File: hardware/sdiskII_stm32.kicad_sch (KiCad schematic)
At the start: 8 parts, among them J2 APPLE_SDISKII, U2 MicroSD_SDIO, U8 DM-OLED096-636

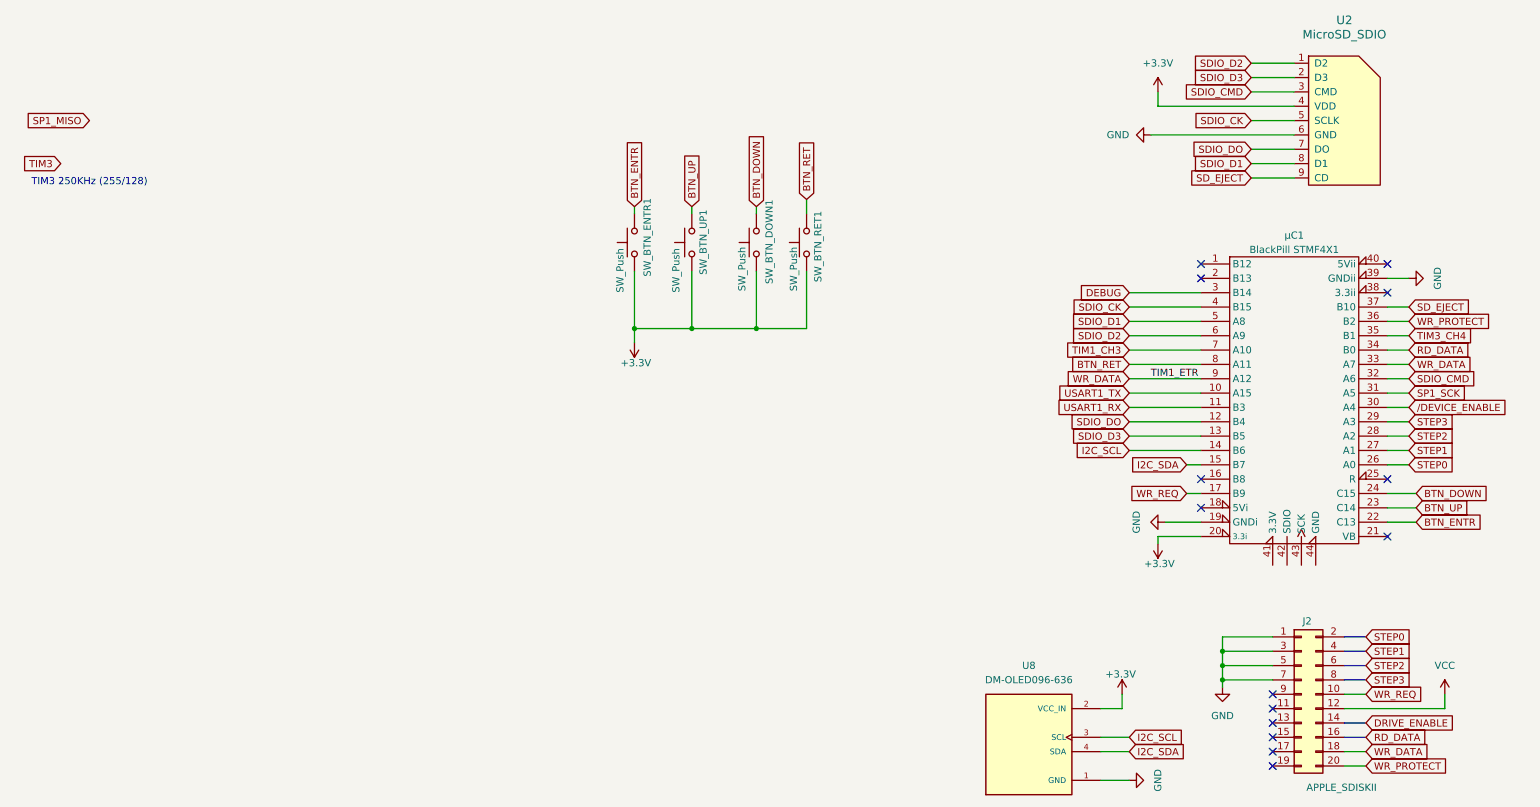
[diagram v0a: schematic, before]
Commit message: new realease with gerber
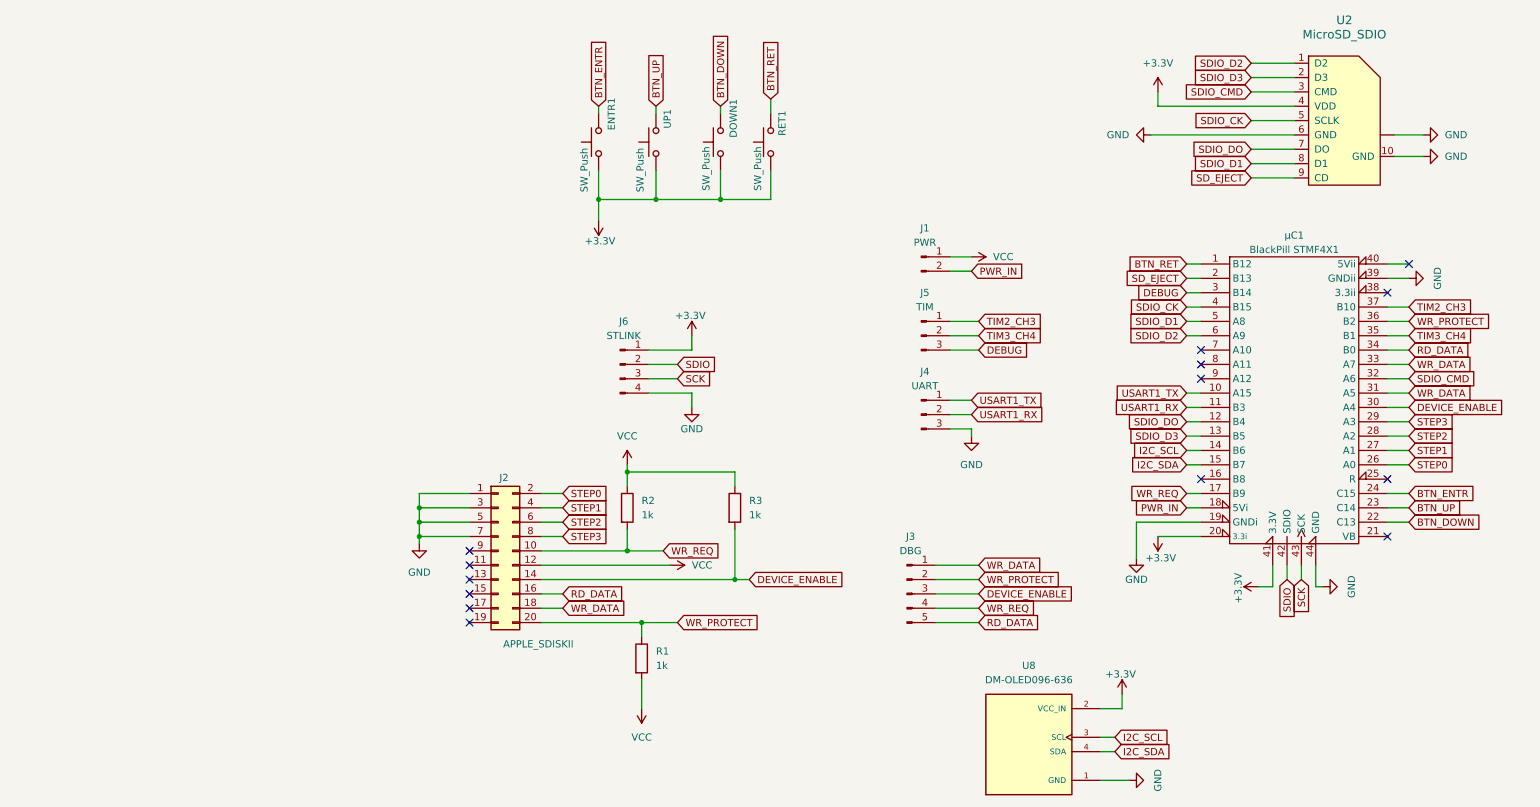
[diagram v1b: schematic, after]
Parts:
- added J1: PWR, Connector_PinHeader_2.54mm:PinHeader_1x02_P2.54mm_Vertical, symbol Connector:Conn_01x02_Pin
- added J3: DBG, Connector_PinHeader_2.54mm:PinHeader_1x05_P2.54mm_Vertical, symbol Connector:Conn_01x05_Pin
- added J4: UART, Connector_PinHeader_2.54mm:PinHeader_1x03_P2.54mm_Vertical, symbol Connector:Conn_01x03_Pin
- added J5: TIM, Connector_PinHeader_2.54mm:PinHeader_1x03_P2.54mm_Vertical, symbol Connector:Conn_01x03_Pin
- added J6: STLINK, Connector_PinHeader_2.54mm:PinHeader_1x04_P2.54mm_Vertical, symbol Connector:Conn_01x04_Pin
- added R1, R2, R3: 1k, Resistor_THT:R_Axial_DIN0207_L6.3mm_D2.5mm_P10.16mm_Horizontal, symbol Device:R
- U2: footprint sdisk_stm32:GCT-MEM2055-00-190-01-A -> sdisk_stm32:GCT-MEM2055-00-190-01-A_VIB
- μC1: footprint acheron_Hardware.pretty-master:Mini_F4X1_STM32 -> acheron_Hardware.pretty-master:Mini_F4X1_STM32_VIB
- renumbered SW_BTN_DOWN1 to DOWN1, SW_BTN_ENTR1 to ENTR1, SW_BTN_RET1 to RET1, SW_BTN_UP1 to UP1
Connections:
- net SP1_SCK is gone; now on net WR_DATA: μC1.31 (A5)
- net /DEVICE_ENABLE is gone; now on net DEVICE_ENABLE: μC1.30 (A4)
- net +3.3V: now also μC1.41 (3.3V), J6.1 (Pin_1)
- net BTN_DOWN: now also μC1.22 (C13); no longer μC1.24 (C15)
- net BTN_ENTR: now also μC1.24 (C15); no longer μC1.22 (C13)
- net BTN_RET: now also μC1.1 (B12); no longer μC1.8 (A11)
- net DEBUG: now also J5.3 (Pin_3)
- net GND: now also U2.10 (GND), U2.~, μC1.44 (GND), J4.3 (Pin_3), J6.4 (Pin_4)
- net RD_DATA: now also J2.16 (Pin_16), J3.5 (Pin_5)
- net SD_EJECT: now also μC1.2 (B13); no longer μC1.37 (B10)
- net STEP0: now also J2.2 (Pin_2)
- net STEP1: now also J2.4 (Pin_4)
- net STEP2: now also J2.6 (Pin_6)
- net STEP3: now also J2.8 (Pin_8)
- net TIM3_CH4: now also J5.2 (Pin_2)
- net USART1_RX: now also J4.2 (Pin_2)
- net USART1_TX: now also J4.1 (Pin_1)
- net VCC: now also J1.1 (Pin_1), R1.2, R2.1, R3.1
- net WR_DATA: now also J3.1 (Pin_1); no longer μC1.9 (A12)
- net WR_PROTECT: now also J3.2 (Pin_2), R1.1
- net WR_REQ: now also J3.4 (Pin_4), R2.2
- net DEVICE_ENABLE: now reaches J2.14 (Pin_14)
- net DEVICE_ENABLE: now also J3.3 (Pin_3), R3.2
- net PWR_IN: now reaches μC1.18 (5Vi)
- net PWR_IN: now also J1.2 (Pin_2)
- net SDIO: now reaches μC1.42 (SDIO)
- net SDIO: now also J6.2 (Pin_2)
- net SCK: now reaches μC1.43 (SCK)
- net SCK: now also J6.3 (Pin_3)
- net TIM1_CH3: no longer names the net of μC1.7 (A10)
- new net TIM2_CH3: J5.1 (Pin_1), μC1.37 (B10)
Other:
- note removed: "TIM3 250KHz (255/128)"
- moved on the sheet: DOWN1, ENTR1, J2, RET1, UP1

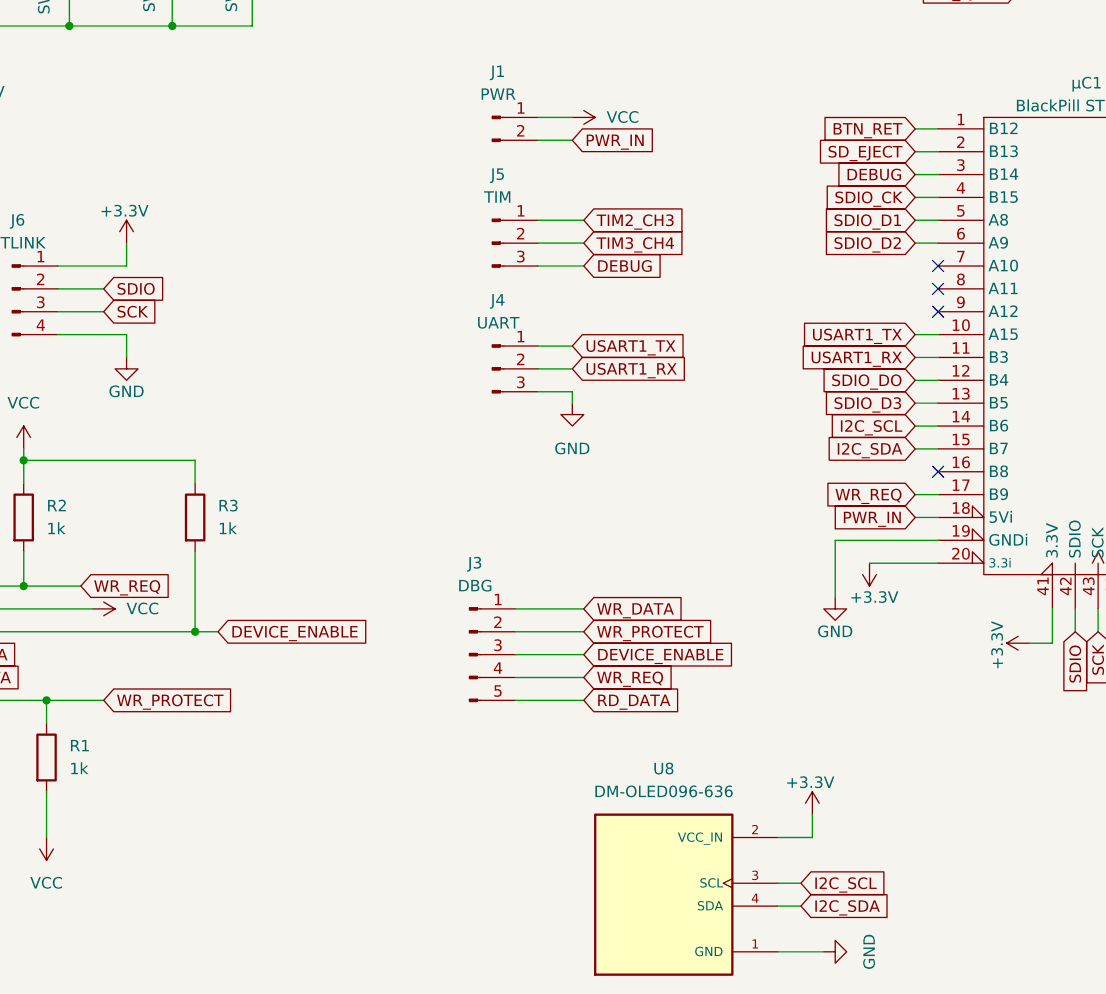
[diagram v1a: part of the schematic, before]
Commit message: board rev20
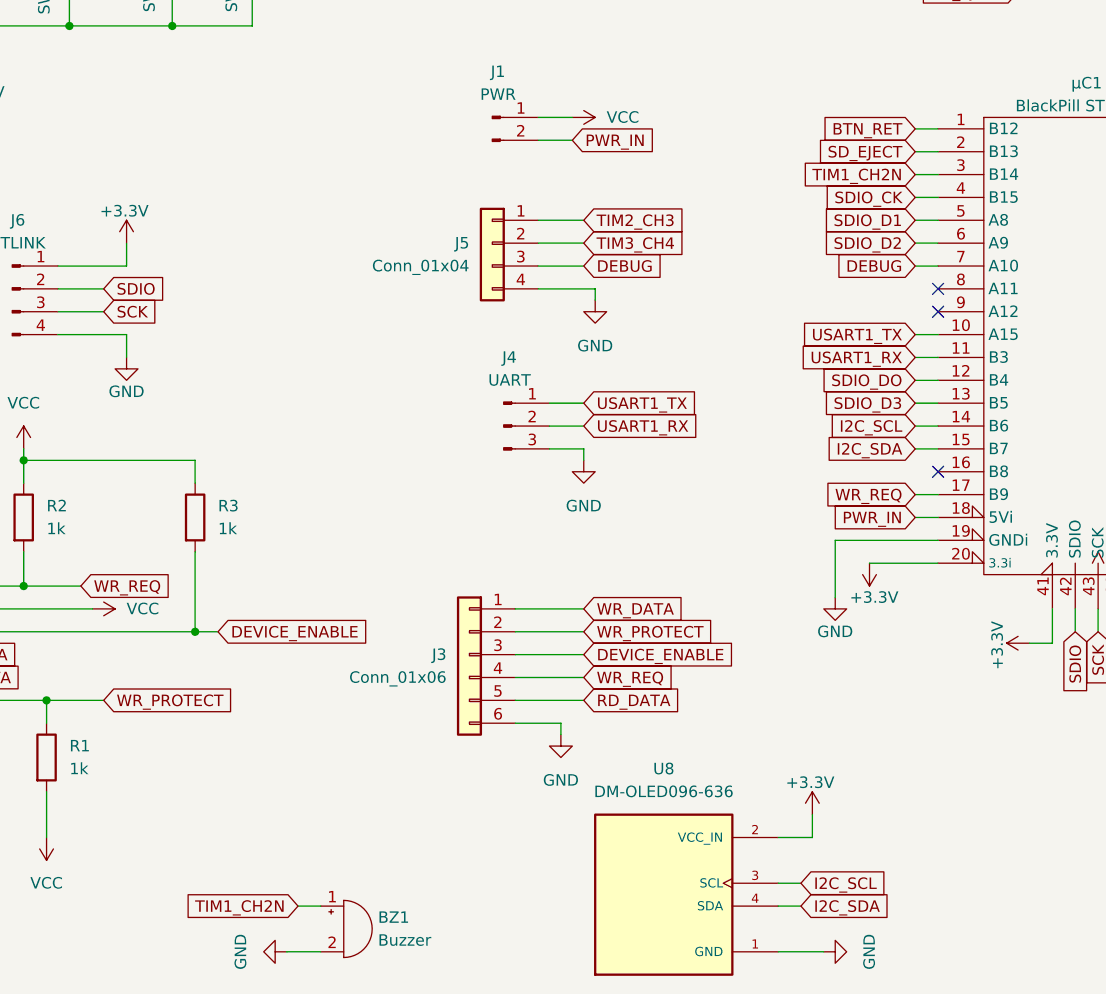
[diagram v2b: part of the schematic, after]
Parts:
- removed J3: DBG, Connector_PinHeader_2.54mm:PinHeader_1x05_P2.54mm_Vertical, symbol Connector:Conn_01x05_Pin
- removed J5: TIM, Connector_PinHeader_2.54mm:PinHeader_1x03_P2.54mm_Vertical, symbol Connector:Conn_01x03_Pin
- added BZ1: Buzzer, symbol Device:Buzzer
- added J3: Conn_01x06, Connector_PinHeader_2.54mm:PinHeader_1x06_P2.54mm_Vertical, symbol Connector_Generic:Conn_01x06
- added J5: Conn_01x04, Connector_PinHeader_2.54mm:PinHeader_1x04_P2.54mm_Vertical, symbol Connector_Generic:Conn_01x04
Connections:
- net DEBUG: now also μC1.7 (A10), J5.3 (Pin_3); no longer μC1.3 (B14)
- net DEVICE_ENABLE: now also J3.3 (Pin_3)
- net GND: now also BZ1.2 (-), J3.6 (Pin_6), J5.4 (Pin_4)
- net RD_DATA: now also J3.5 (Pin_5)
- net TIM2_CH3: now also J5.1 (Pin_1)
- net TIM3_CH4: now also J5.2 (Pin_2)
- net WR_DATA: now also J3.1 (Pin_1)
- net WR_PROTECT: now also J3.2 (Pin_2)
- net WR_REQ: now also J3.4 (Pin_4)
- new net TIM1_CH2N: BZ1.1 (+), μC1.3 (B14)
- no-connect marks 14 -> 13
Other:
- moved on the sheet: J4

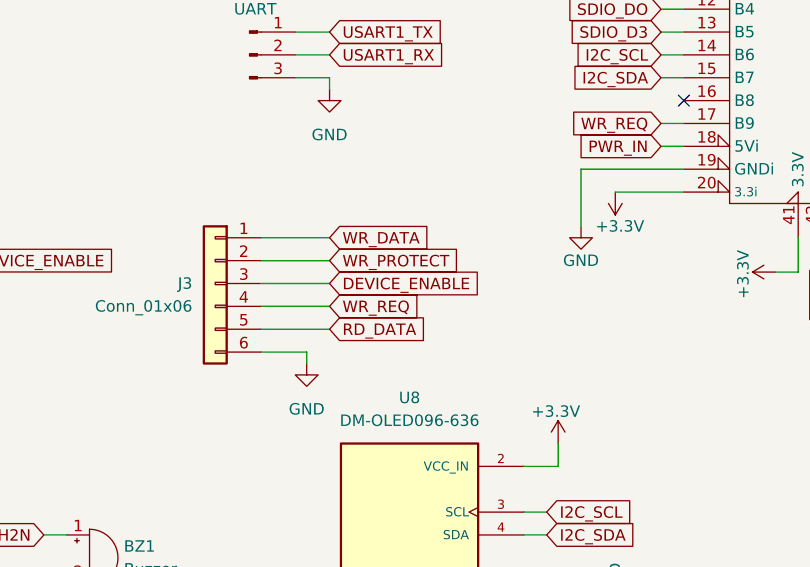
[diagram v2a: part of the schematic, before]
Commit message: board rev2
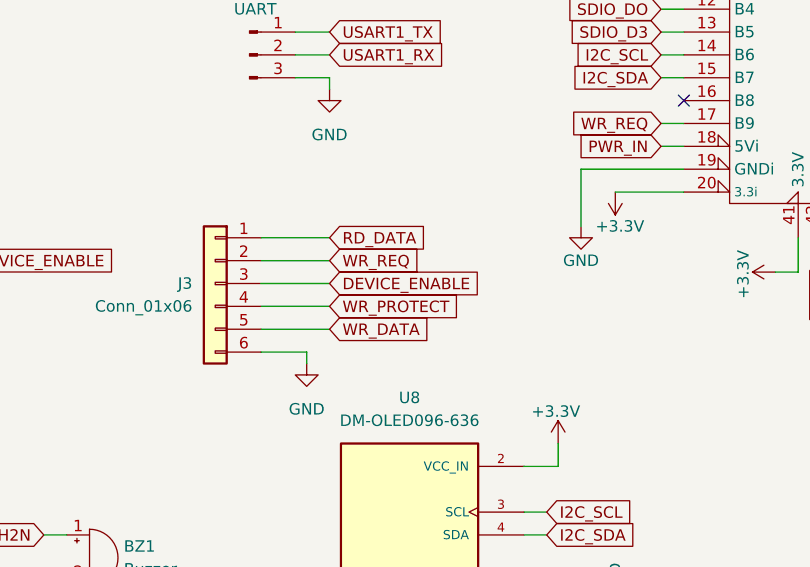
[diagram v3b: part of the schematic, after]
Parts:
- BZ1: footprint (none) -> buzzer:AS-1201B-LF
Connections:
- net RD_DATA: now also J3.1 (Pin_1); no longer J3.5 (Pin_5)
- net WR_DATA: now also J3.5 (Pin_5); no longer J3.1 (Pin_1)
- net WR_PROTECT: now also J3.4 (Pin_4); no longer J3.2 (Pin_2)
- net WR_REQ: now also J3.2 (Pin_2); no longer J3.4 (Pin_4)
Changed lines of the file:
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@@
 	(wire
 		(pts
-			(xy 124.46 80.01) (xy 129.54 80.01)
+			(xy 175.26 113.03) (xy 182.88 113.03)
 		)
 		(stroke
@@
 	(wire
 		(pts
-			(xy 137.16 48.26) (xy 146.05 48.26)
+			(xy 124.46 80.01) (xy 129.54 80.01)
 		)
 		(stroke
@@
 	(wire
 		(pts
-			(xy 219.71 95.25) (xy 222.25 95.25)
+			(xy 137.16 48.26) (xy 146.05 48.26)
 		)
 		(stroke
@@
 	(wire
 		(pts
-			(xy 255.27 102.87) (xy 259.08 102.87)
+			(xy 219.71 95.25) (xy 222.25 95.25)
 		)
 		(stroke
@@
 	(wire
 		(pts
-			(xy 105.41 102.87) (xy 109.22 102.87)
+			(xy 255.27 102.87) (xy 259.08 102.87)
 		)
 		(stroke
@@
 	(wire
 		(pts
-			(xy 219.71 59.69) (xy 222.25 59.69)
+			(xy 105.41 102.87) (xy 109.22 102.87)
 		)
 		(stroke
@@
 	(wire
 		(pts
-			(xy 175.26 115.57) (xy 182.88 115.57)
+			(xy 219.71 59.69) (xy 222.25 59.69)
 		)
 		(stroke
@@
 	(wire
 		(pts
-			(xy 175.26 120.65) (xy 182.88 120.65)
-		)
-		(stroke
-			(width 0)
-			(type default)
-		)
-	)
-	(wire
-		(pts
 			(xy 182.88 95.25) (xy 182.88 96.52)
 		)
@@
 	(wire
 		(pts
+			(xy 175.26 115.57) (xy 182.88 115.57)
+		)
+		(stroke
+			(width 0)
+			(type default)
+		)
+	)
+	(wire
+		(pts
 			(xy 175.26 125.73) (xy 180.34 125.73)
 		)
@@
 	(wire
 		(pts
+			(xy 175.26 123.19) (xy 182.88 123.19)
+		)
+		(stroke
+			(width 0)
+			(type default)
+		)
+	)
+	(wire
+		(pts
 			(xy 146.05 43.18) (xy 146.05 48.26)
 		)
@@
 	(wire
 		(pts
-			(xy 256.54 36.83) (xy 261.62 36.83)
+			(xy 175.26 120.65) (xy 182.88 120.65)
 		)
 		(stroke
@@
 	(wire
 		(pts
-			(xy 231.14 26.67) (xy 238.76 26.67)
+			(xy 256.54 36.83) (xy 261.62 36.83)
 		)
 		(stroke
@@
 	(wire
 		(pts
-			(xy 255.27 74.93) (xy 259.08 74.93)
+			(xy 231.14 26.67) (xy 238.76 26.67)
 		)
 		(stroke
@@
 	(wire
 		(pts
-			(xy 175.26 113.03) (xy 182.88 113.03)
+			(xy 255.27 74.93) (xy 259.08 74.93)
 		)
 		(stroke
@@
 	(wire
 		(pts
-			(xy 175.26 123.19) (xy 182.88 123.19)
-		)
-		(stroke
-			(width 0)
-			(type default)
-		)
-	)
-	(wire
-		(pts
 			(xy 105.41 115.57) (xy 139.7 115.57)
 		)
@@
 	(global_label "WR_DATA"
 		(shape input)
-		(at 182.88 113.03 0)
+		(at 182.88 123.19 0)
 		(fields_autoplaced yes)
 		(effects
@@
 		)
 		(property "Intersheetrefs" "${INTERSHEET_REFS}"
-			(at 193.969 113.03 0)
+			(at 193.969 123.19 0)
 			(effects
 				(font
@@
 	(global_label "WR_PROTECT"
 		(shape input)
-		(at 182.88 115.57 0)
+		(at 182.88 120.65 0)
 		(fields_autoplaced yes)
 		(effects
@@
 		)
 		(property "Intersheetrefs" "${INTERSHEET_REFS}"
-			(at 197.7789 115.57 0)
+			(at 197.7789 120.65 0)
 			(effects
 				(font
@@
 	(global_label "WR_REQ"
 		(shape input)
-		(at 182.88 120.65 0)
+		(at 182.88 115.57 0)
 		(fields_autoplaced yes)
 		(effects
@@
 		)
 		(property "Intersheetrefs" "${INTERSHEET_REFS}"
-			(at 193.3037 120.65 0)
+			(at 193.3037 115.57 0)
 			(effects
 				(font
@@
 	(global_label "RD_DATA"
 		(shape input)
-		(at 182.88 123.19 0)
+		(at 182.88 113.03 0)
 		(fields_autoplaced yes)
 		(effects
@@
 		)
 		(property "Intersheetrefs" "${INTERSHEET_REFS}"
-			(at 193.7876 123.19 0)
+			(at 193.7876 113.03 0)
 			(effects
 				(font
@@
 			)
 		)
-		(property "Footprint" ""
+		(property "Footprint" "buzzer:AS-1201B-LF"
 			(at 155.575 146.05 90)
 			(effects
